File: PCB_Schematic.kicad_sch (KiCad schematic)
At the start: 47 parts, among them J1 IMU_1, J2 Power_Connector, J3 Conn_02x05_Odd_Even, J6 USB_A, J7 Ultrasonic, J8 IMU_2, Q7 BSS138, SW1 SW_Push, U2 LM1117MP-ADJ, U3 TPS54331-Q1, U5 FT232RL, U6 STM32F091RCTx

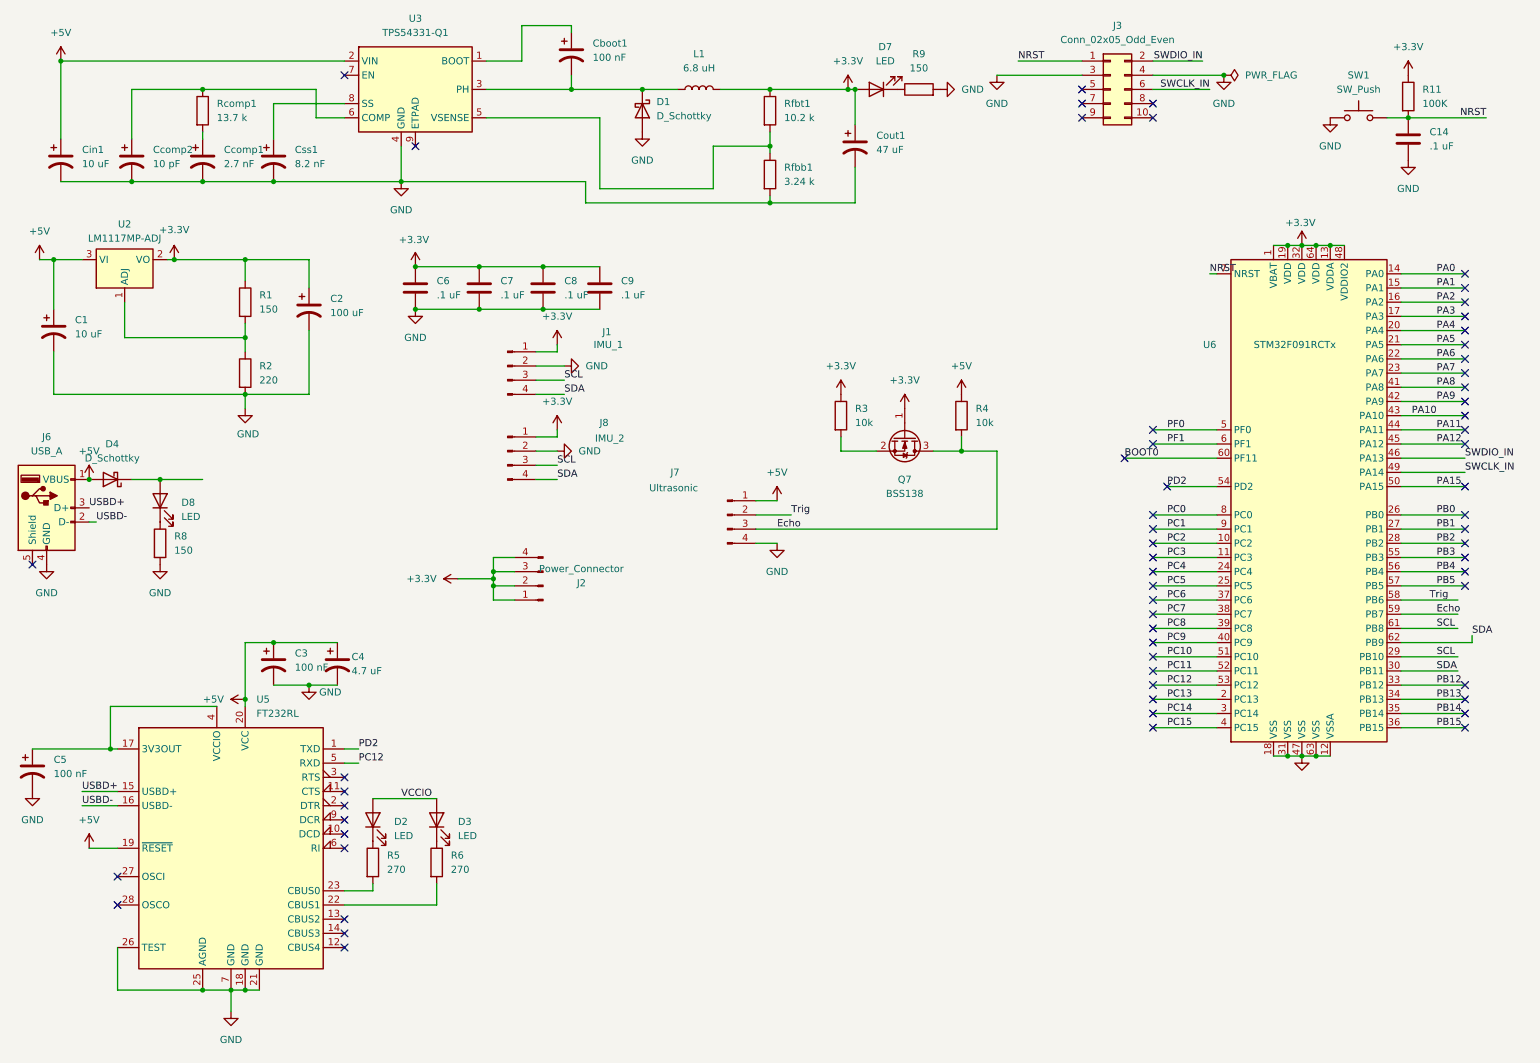
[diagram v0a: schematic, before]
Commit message: Sam
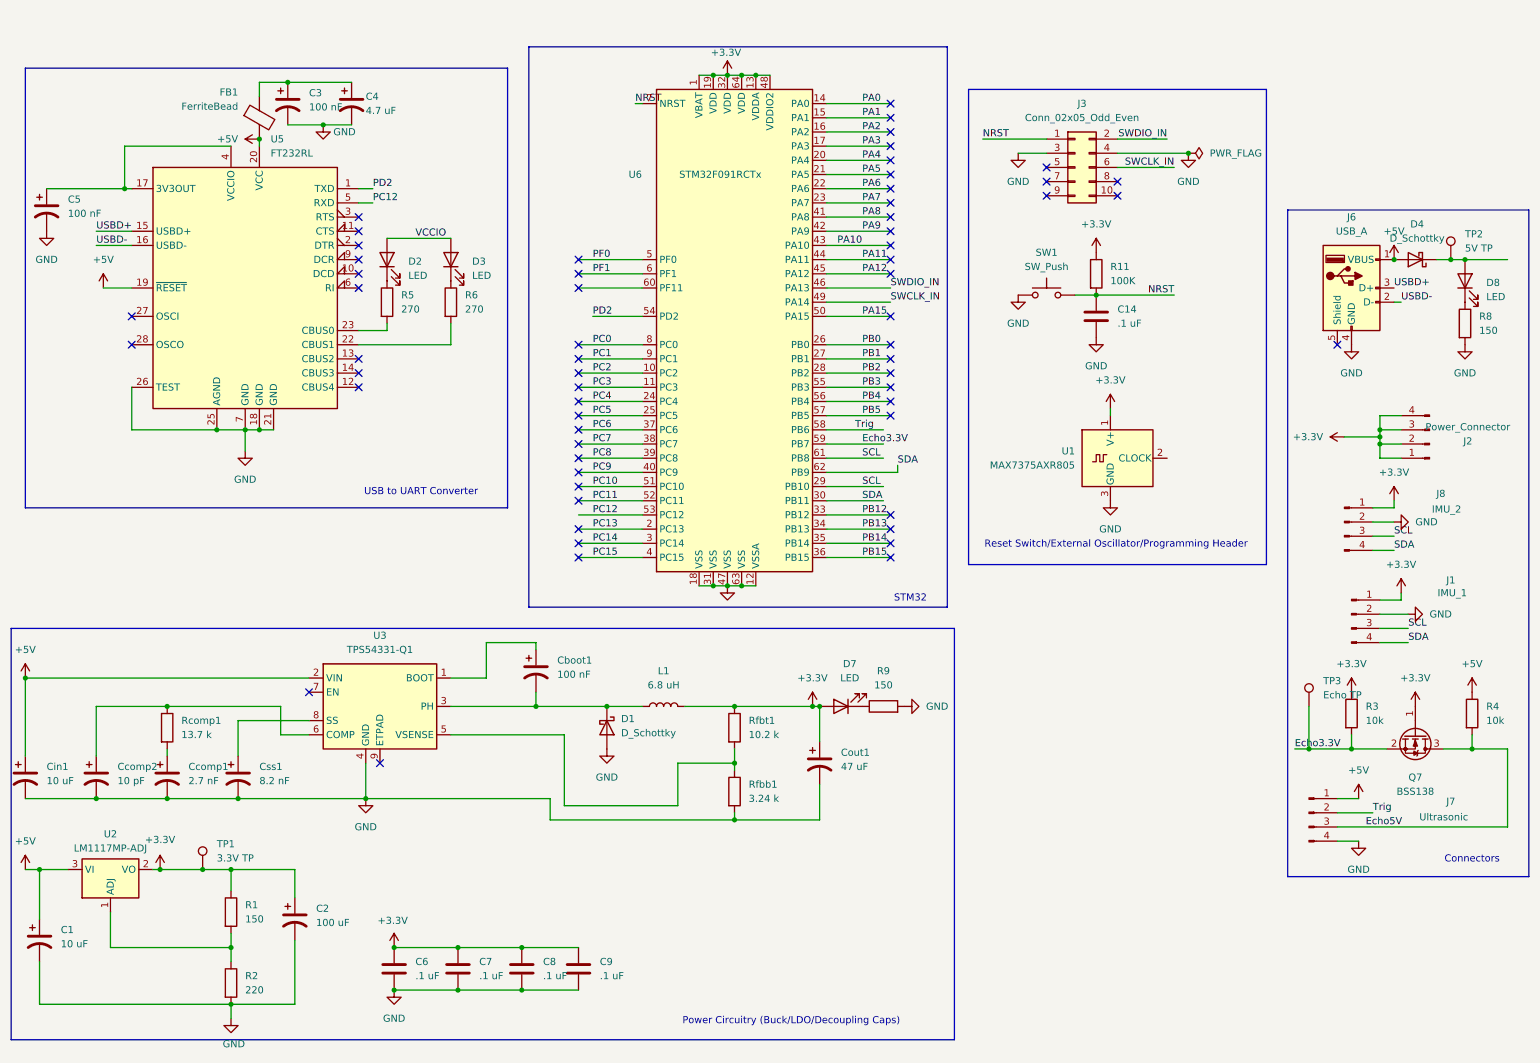
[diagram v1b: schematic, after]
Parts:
- added FB1: FerriteBead, Inductor_SMD:L_0201_0603Metric_Pad0.64x0.40mm_HandSolder, symbol Device:FerriteBead
- added TP1: 3.3V TP, symbol Connector:TestPoint
- added TP2: 5V TP, symbol Connector:TestPoint
- added TP3: Echo TP, symbol Connector:TestPoint
- added U1: MAX7375AXR805, Package_TO_SOT_SMD:SOT-323_SC-70, symbol Oscillator:MAX7375AXR805
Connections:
- net +3.3V: now also TP1.1, U1.1 (V+)
- net +5V: now also FB1.2; no longer C3.1, C4.1
- net GND: now also U1.3 (GND)
- net Echo3.3V: now reaches Q7.2 (S), R3.2
- net Echo3.3V: now also U6.59 (PB7), TP3.1
- net at D4.1 (K), D8.2 (A): now also TP2.1
- net BOOT0: no longer names the net of U6.60 (PF11)
- net Echo renamed Echo5V
- net Echo5V: no longer U6.59 (PB7)
- new net: C3.1, C4.1, FB1.1
- no-connect marks 63 -> 61
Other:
- note added: "Connectors"
- note added: "Power Circuitry (Buck/LDO/Decoupling Caps)"
- note added: "Reset Switch/External Oscillator/Programming Header"
- note added: "STM32"
- note added: "USB to UART Converter"
- moved on the sheet: C1, C14, C2, C3, C4, C5, C6, C7, C8, C9, Cboot1, Ccomp1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
